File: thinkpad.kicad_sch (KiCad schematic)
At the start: 126 parts, among them J1 Conn_01x06_MountingPin, J2 Conn_01x20_Socket, J3 Conn_01x06_Socket, J4 Touchpad_Conn, U1 Raspberry_Pi_Pico

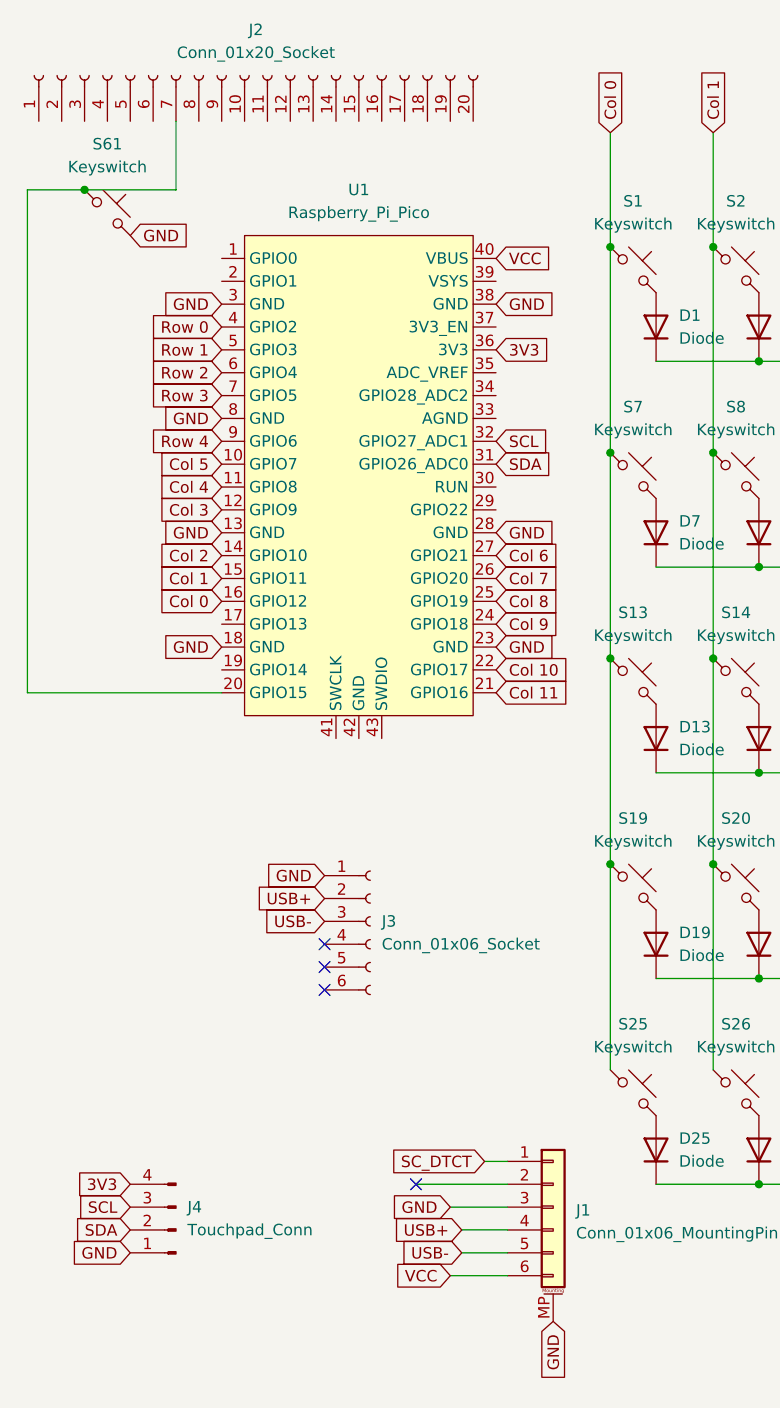
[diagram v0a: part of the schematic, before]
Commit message: Change switches
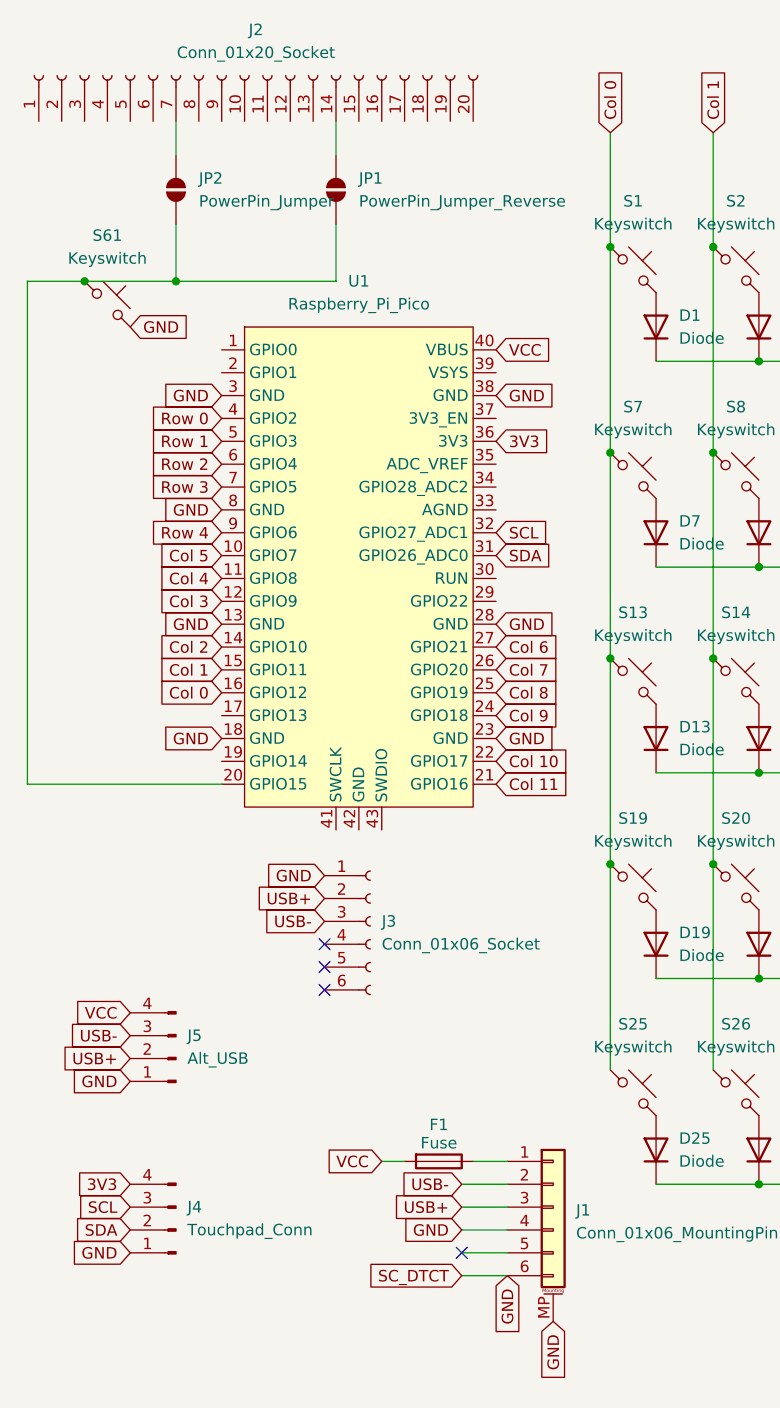
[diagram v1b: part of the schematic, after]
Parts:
- added F1: Fuse, Fuse:Fuse_0805_2012Metric, symbol Device:Fuse
- added J5: Alt_USB, Connector_PinHeader_2.54mm:PinHeader_1x04_P2.54mm_Vertical, symbol Connector:Conn_01x04_Pin
- added JP1: PowerPin_Jumper_Reverse, Jumper:SolderJumper-2_P1.3mm_Open_Pad1.0x1.5mm, symbol Jumper:SolderJumper_2_Open
- added JP2: PowerPin_Jumper, Jumper:SolderJumper-2_P1.3mm_Open_Pad1.0x1.5mm, symbol Jumper:SolderJumper_2_Open
- D1, D10, D11, D12, D13, D14, D15, D16, D17, D18, D19, D2, D20, D21, D22, D23, D24, D25, D26, D27, D28, D29, D3, D30, D31, D32, D33, D34, D35, D36, D37, D38, D39, D4, D40, D41, D42, D43, D44, D45, D46, D47, D48, D49, D5, D50, D51, D52, D53, D54, D55, D56, D57, D58, D59, D6, D60, D7, D8, D9: footprint ScottoKeebs_Components:Diode_DO-35 -> thinkpad-keyboard:Diode_SMD_THT2
- S1, S10, S11, S12, S13, S14, S15, S16, S17, S18, S19, S2, S20, S21, S22, S23, S24, S25, S26, S27, S28, S29, S3, S30, S31, S32, S33, S34, S35, S36, S37, S38, S39, S4, S40, S41, S42, S43, S44, S45, S46, S47, S48, S49, S5, S50, S51, S52, S53, S54, S55, S56, S57, S58, S59, S6, S60, S61, S7, S8, S9: footprint ScottoKeebs_Choc:Choc_Mini_1.00u -> kailh-pg1425-x-switch:Kailh-PG1425-X-Switch
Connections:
- net GND: now also J1.4 (Pin_4), J1.6 (Pin_6), J5.1 (Pin_1); no longer J1.3 (Pin_3)
- net USB+: now also J1.3 (Pin_3), J5.2 (Pin_2); no longer J1.4 (Pin_4)
- net USB-: now also J1.2 (Pin_2), J5.3 (Pin_3); no longer J1.5 (Pin_5)
- net VCC: now also F1.2, J5.4 (Pin_4); no longer J1.6 (Pin_6)
- net at S61.1, U1.20 (GPIO15): now also JP1.1 (A), JP2.1 (A); no longer J2.7 (Pin_7)
- net at J2.14 (Pin_14): now also JP1.2 (B)
- net SC_DTCT: no longer names the net of J1.1 (Pin_1)
- net SC_DTCT: now also F1.1
- new net: J2.7 (Pin_7), JP2.2 (B)
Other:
- moved on the sheet: S61, U1
